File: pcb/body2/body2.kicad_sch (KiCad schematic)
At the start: 17 parts, among them J1 FRETBOARD_CONNECTION, J2 Conn_01x20_Pin, J4 Conn_01x10, U1 Teensy4.1, U2 TCA9548APWR

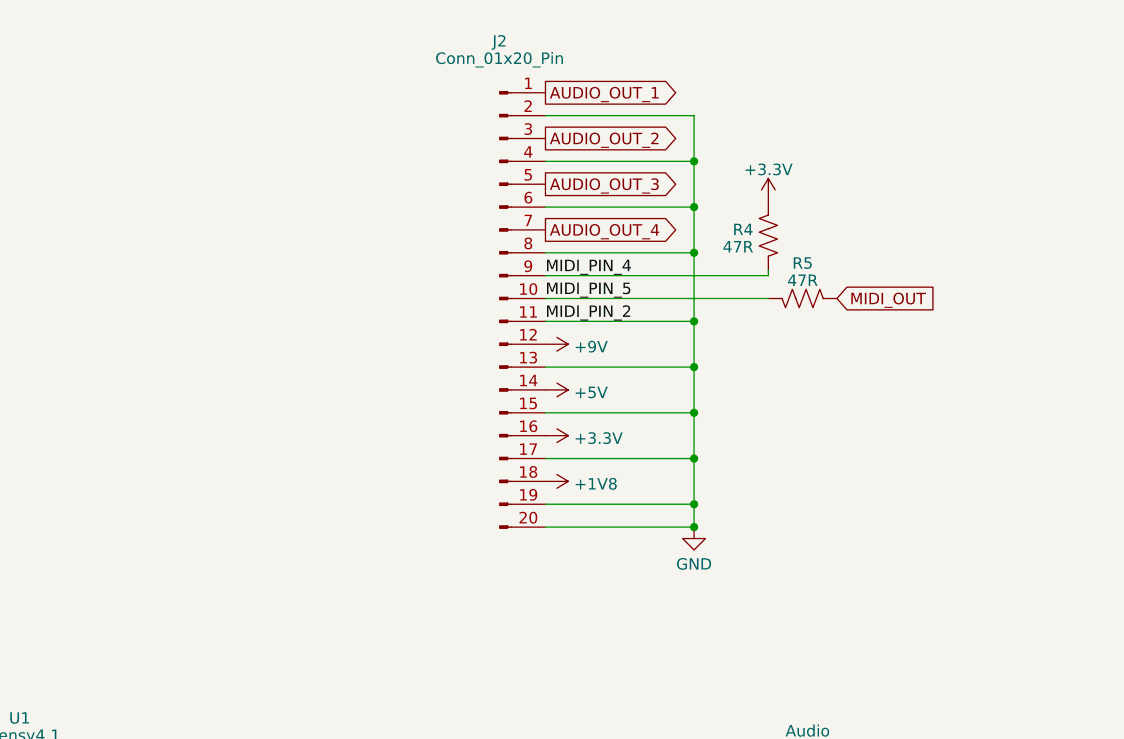
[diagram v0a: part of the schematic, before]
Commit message: nicer layout
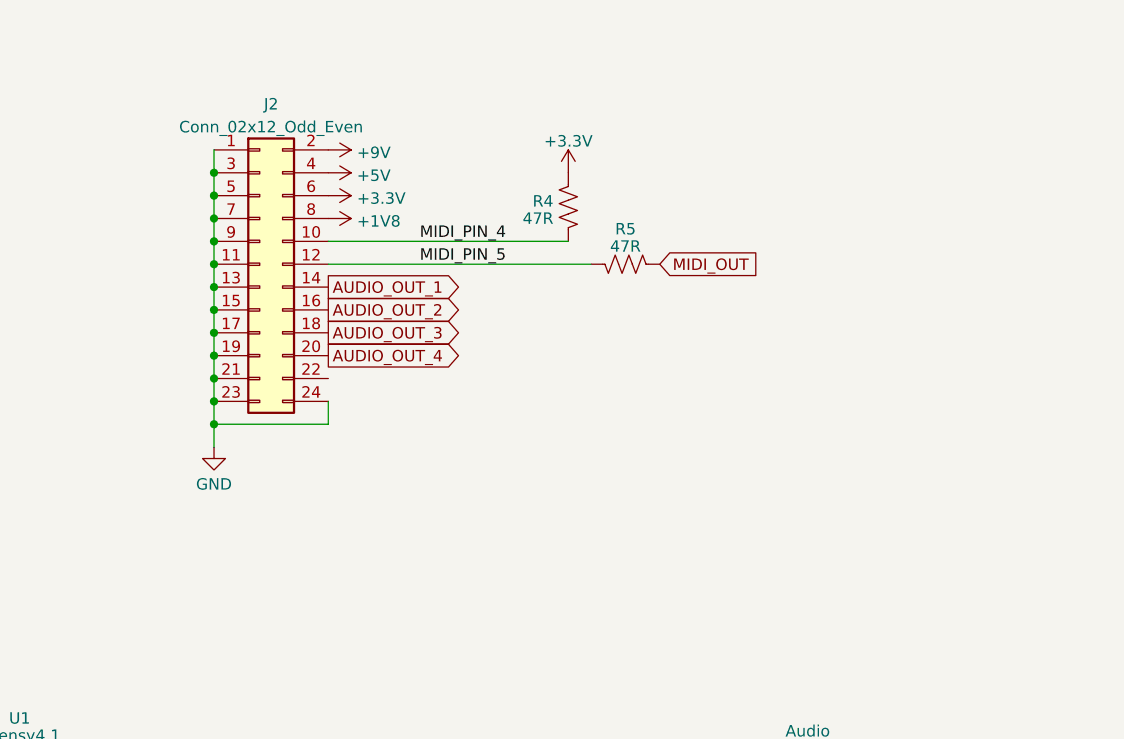
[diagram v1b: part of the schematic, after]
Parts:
- removed J2: Conn_01x20_Pin, Connector_PinHeader_2.54mm:PinHeader_1x20_P2.54mm_Vertical, symbol Connector:Conn_01x20_Pin
- added J2: Conn_02x12_Odd_Even, Connector_PinHeader_2.54mm:PinHeader_2x12_P2.54mm_Vertical, symbol Connector_Generic:Conn_02x12_Odd_Even
- J4: footprint Connector_PinHeader_2.54mm:PinHeader_1x10_P2.54mm_Vertical -> Connector_PinHeader_1.27mm:PinHeader_1x10_P1.27mm_Vertical
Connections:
- net +1V8: now also J2.8 (Pin_8)
- net +3.3V: now also J2.6 (Pin_6)
- net +5V: now also J2.4 (Pin_4)
- net +9V: now also J2.2 (Pin_2)
- net AUDIO_OUT_1: now also J2.14 (Pin_14)
- net AUDIO_OUT_2: now also J2.16 (Pin_16)
- net AUDIO_OUT_3: now also J2.18 (Pin_18)
- net AUDIO_OUT_4: now also J2.20 (Pin_20)
- net GND: now also J2.1 (Pin_1), J2.11 (Pin_11), J2.13 (Pin_13), J2.15 (Pin_15), J2.17 (Pin_17), J2.19 (Pin_19), J2.21 (Pin_21), J2.23 (Pin_23), J2.24 (Pin_24), J2.3 (Pin_3), J2.5 (Pin_5), J2.7 (Pin_7), J2.9 (Pin_9)
- net MIDI_PIN_4: now also J2.10 (Pin_10)
- net MIDI_PIN_5: now also J2.12 (Pin_12)
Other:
- moved on the sheet: R4, R5
